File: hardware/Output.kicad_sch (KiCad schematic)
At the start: 9 parts, among them Q501 2N7002, Q502 AO4407A

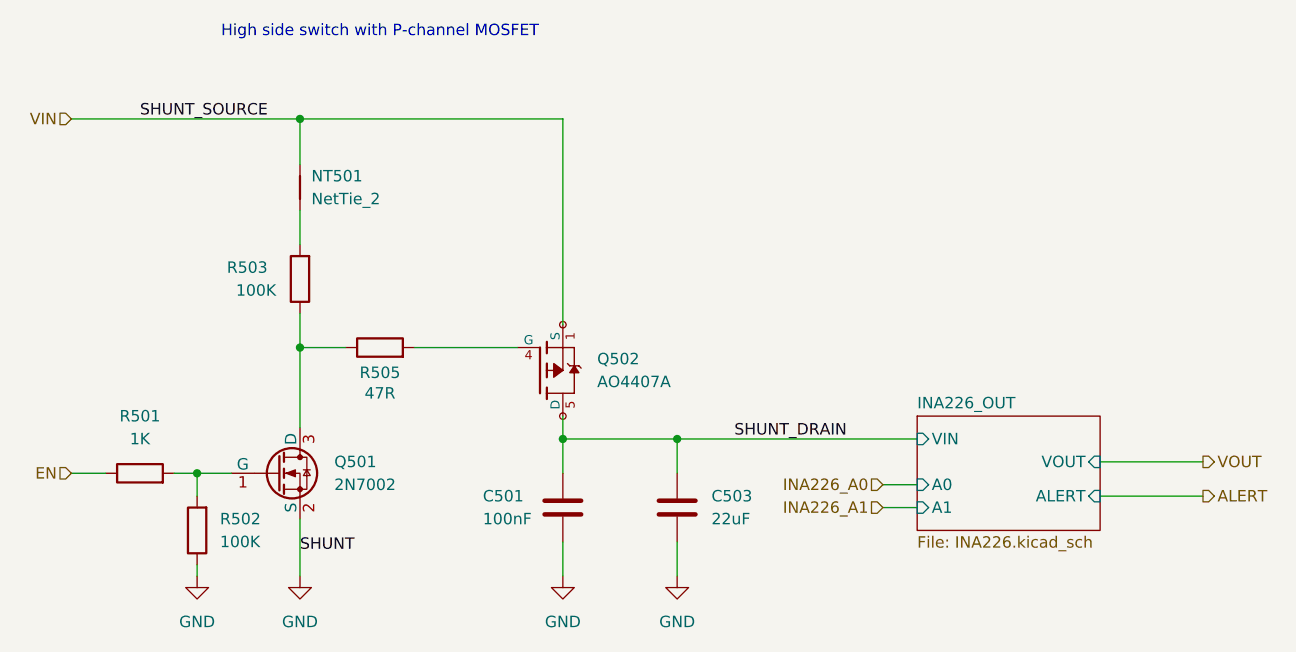
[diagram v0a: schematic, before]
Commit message: PWR_FLG
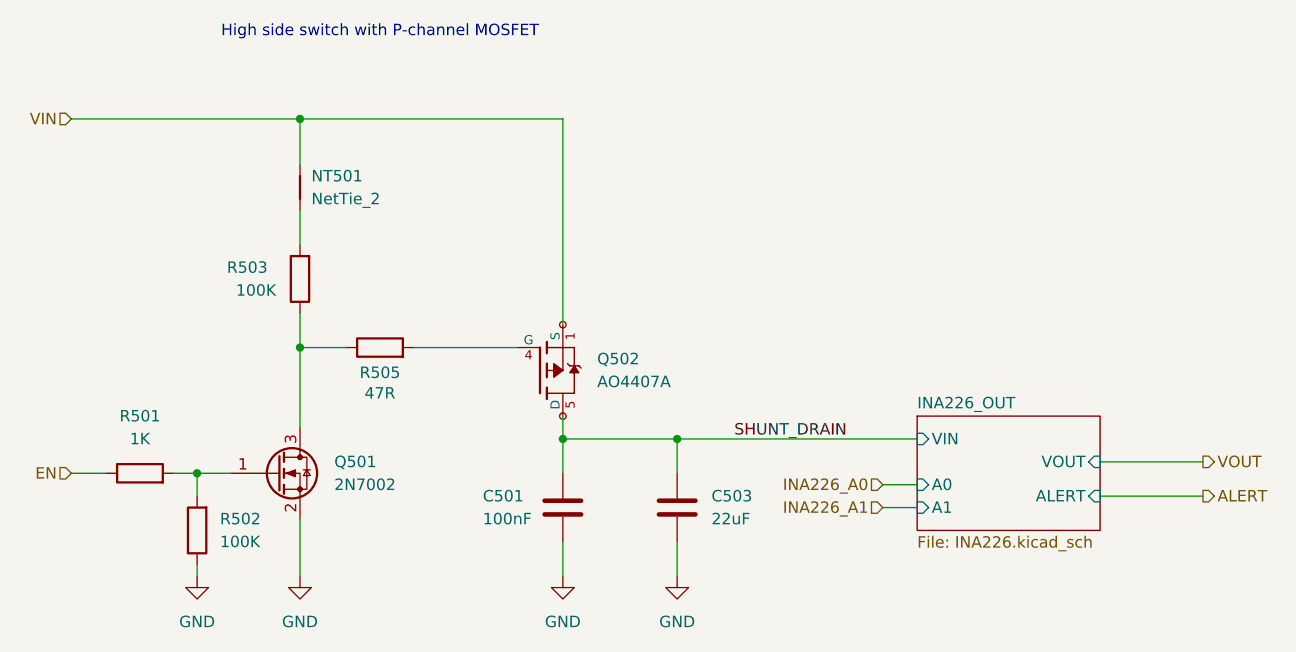
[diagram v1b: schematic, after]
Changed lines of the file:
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@@
-		)
-	)
-	(label "SHUNT"
-		(at 77.47 113.03 0)
-		(effects
-			(font
-				(size 1.27 1.27)
-			)
-			(justify left bottom)
-		)
-	)
-	(label "SHUNT_SOURCE"
-		(at 59.69 64.77 0)
-		(effects
-			(font
-				(size 1.27 1.27)
-			)
-			(justify left bottom)
 		)
 	)
